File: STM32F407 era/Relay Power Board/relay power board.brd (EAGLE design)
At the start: 135.9 x 58.4 mm, 37 parts, among them X1 5566-6, X2 22-23-2031, X3 22-23-2021, X4 22-23-2021

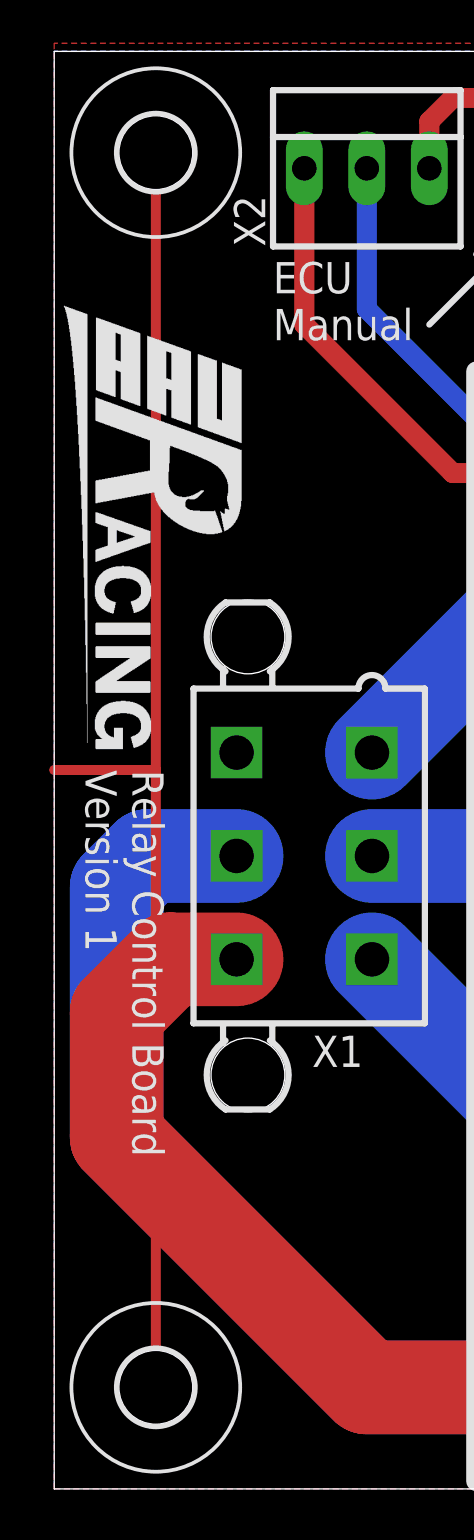
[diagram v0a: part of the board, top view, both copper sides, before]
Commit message: All boards RC done!
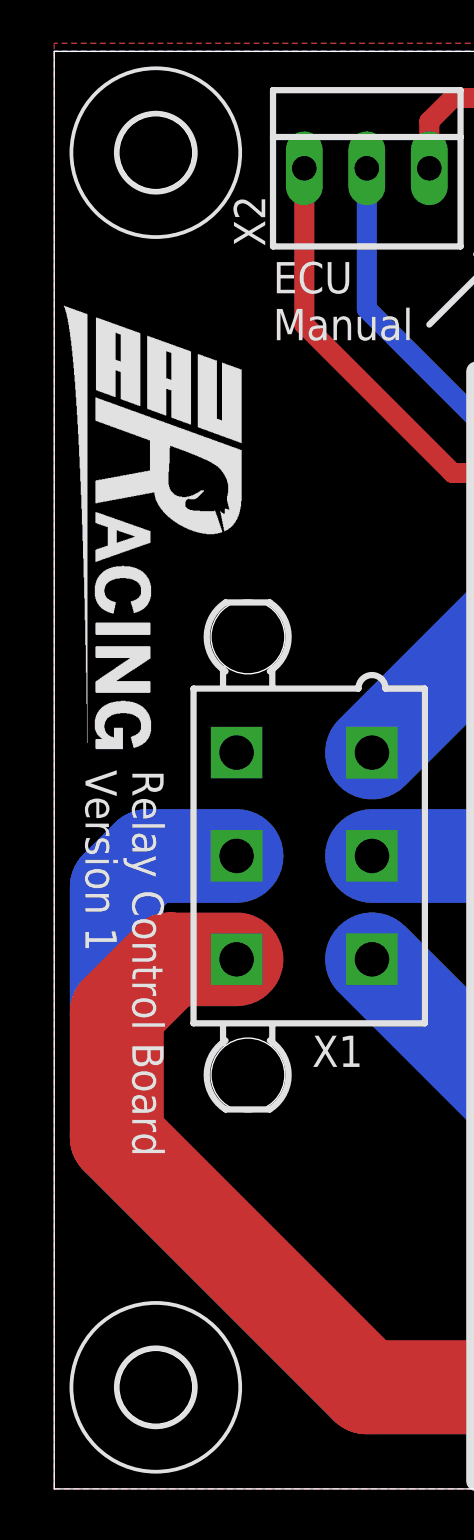
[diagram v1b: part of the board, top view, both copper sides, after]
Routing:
- net N$27: track 54.3 -> 0.00 mm
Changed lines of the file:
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@@
 Version 1</text>
 <wire x1="15.24" y1="47.3075" x2="18.0975" y2="50.165" width="0.254" layer="112"/>
-<dimension x1="0" y1="58.42" x2="0" y2="0" x3="-7.62" y3="29.21" layer="1"/>
-<dimension x1="135.89" y1="58.7375" x2="0" y2="58.7375" x3="67.945" y3="69.5325" layer="1"/>
-<dimension x1="0" y1="0" x2="0" y2="29.21" x3="-7.62" y3="14.605" layer="1"/>
-<dimension x1="4.1275" y1="29.21" x2="4.1275" y2="54.2925" x3="-2.2225" y3="41.75125" layer="1"/>
-<dimension x1="4.1275" y1="4.1275" x2="4.1275" y2="29.21" x3="-2.2225" y3="16.66875" layer="1"/>
-<dimension x1="0" y1="29.21" x2="4.1275" y2="29.21" x3="2.06375" y3="62.865" layer="1"/>
 <wire x1="4.1275" y1="29.21" x2="132.08" y2="29.21" width="0.4064" layer="37"/>
 <wire x1="132.08" y1="29.21" x2="132.08" y2="54.2925" width="0.4064" layer="37"/>
@@
 </signal>
 <signal name="N$27">
-<wire x1="0" y1="29.21" x2="4.1275" y2="29.21" width="0.4064" layer="1"/>
-<wire x1="4.1275" y1="29.21" x2="4.1275" y2="54.2925" width="0.4064" layer="1"/>
-<wire x1="4.1275" y1="4.1275" x2="4.1275" y2="29.21" width="0.4064" layer="1"/>
 </signal>
 </signals>
